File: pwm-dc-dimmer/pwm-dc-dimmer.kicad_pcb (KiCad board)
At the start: 2 copper layers, 61 x 125.5 mm, 90 parts, among them J1 Screw_Terminal_01x02, J10 Screw_Terminal_01x02, J11 Screw_Terminal_01x02, J12 Screw_Terminal_01x02, J13 Screw_Terminal_01x02, J14 Conn_02x03_Odd_Even, J15 Conn_02x03_Odd_Even, J2 Screw_Terminal_01x02, J3 Screw_Terminal_01x02, J4 Screw_Terminal_01x02, J5 Screw_Terminal_01x02, J6 Screw_Terminal_01x02, J7 Screw_Terminal_01x02, J8 Screw_Terminal_01x02, J9 Screw_Terminal_01x02, Q1 Q_NMOS_GDS, Q10 Q_NMOS_GDS, Q11 Q_NMOS_GDS, Q12 Q_NMOS_GDS, Q2 Q_NMOS_GDS, Q3 Q_NMOS_GDS, Q4 Q_NMOS_GDS, Q5 Q_NMOS_GDS, Q6 Q_NMOS_GDS, Q7 Q_NMOS_GDS, Q8 Q_NMOS_GDS, Q9 Q_NMOS_GDS

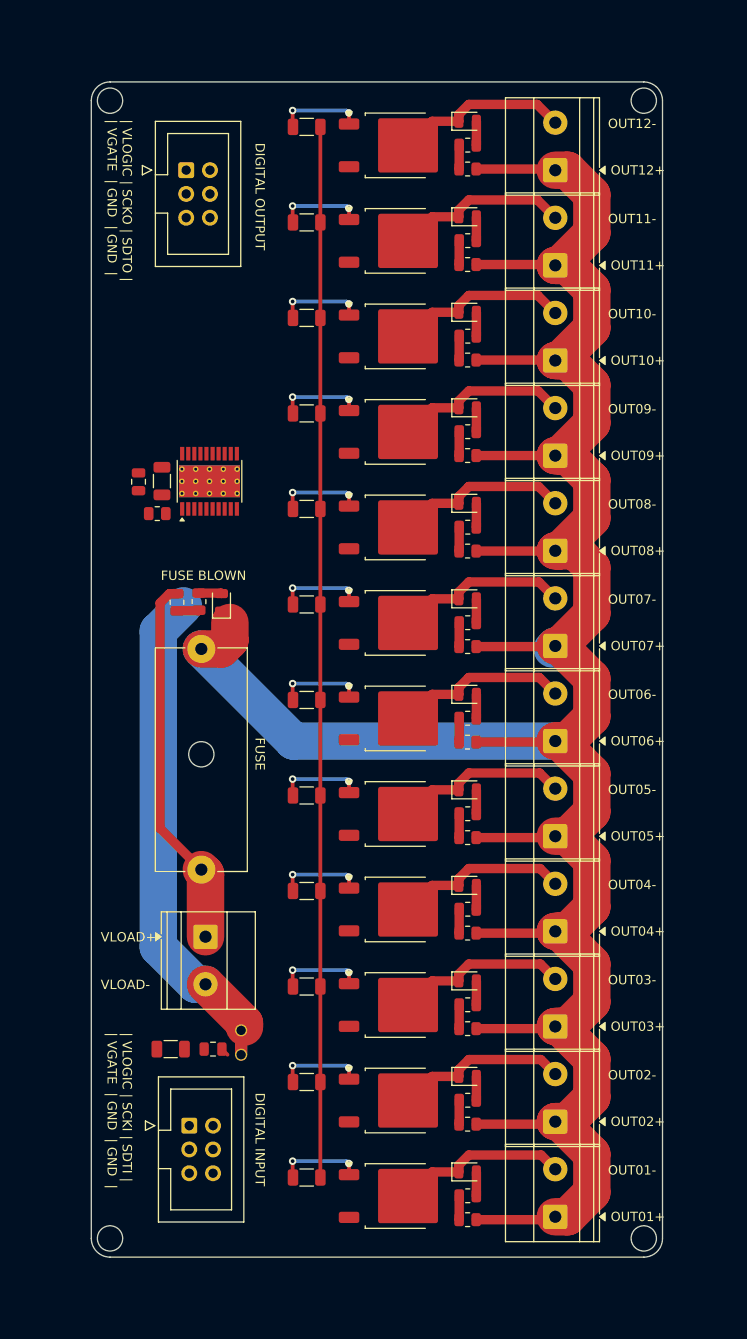
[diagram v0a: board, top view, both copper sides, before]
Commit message: Finish routing
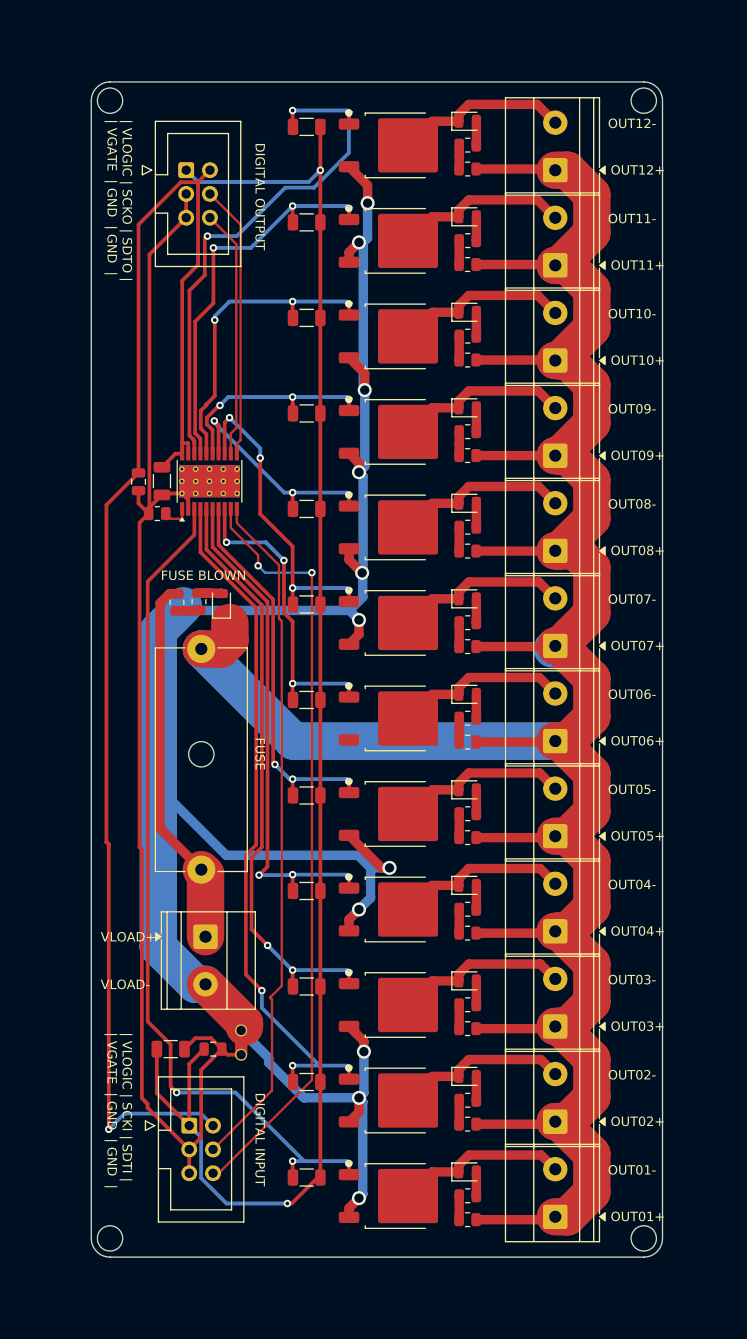
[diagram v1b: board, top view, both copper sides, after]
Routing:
- net GND_LOAD: track 50.5 -> 218.4 mm, vias 0 -> 11
- net GND: track 0.85 -> 157.0 mm
- net V_LOGIC: track 0.00 -> 155.1 mm, vias 0 -> 1
- net GATE_SINK_1: track 9.07 -> 91.9 mm, vias 2 -> 3
- net SDTI: track 0.00 -> 82.2 mm, vias 0 -> 2
- net SCKI: track 0.00 -> 73.8 mm
- net GATE_SINK_2: track 9.07 -> 74.7 mm, vias 2 -> 3
- net V_GATE: track 113.1 -> 173.4 mm, vias 0 -> 2
- net GATE_SINK_3: track 9.07 -> 63.1 mm, vias 2 -> 3
- net GATE_SINK_12: track 9.07 -> 56.6 mm, vias 2 -> 3
- net GATE_SINK_4: track 9.07 -> 55.1 mm, vias 2 -> 3
- net GATE_SINK_11: track 9.07 -> 42.4 mm, vias 2 -> 3
- net GATE_SINK_5: track 9.07 -> 41.4 mm, vias 2 -> 3
- net SCKO: track 0.00 -> 29.3 mm
- net SDTO: track 0.00 -> 26.6 mm
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
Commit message: Finalize DC dimmer v0.1
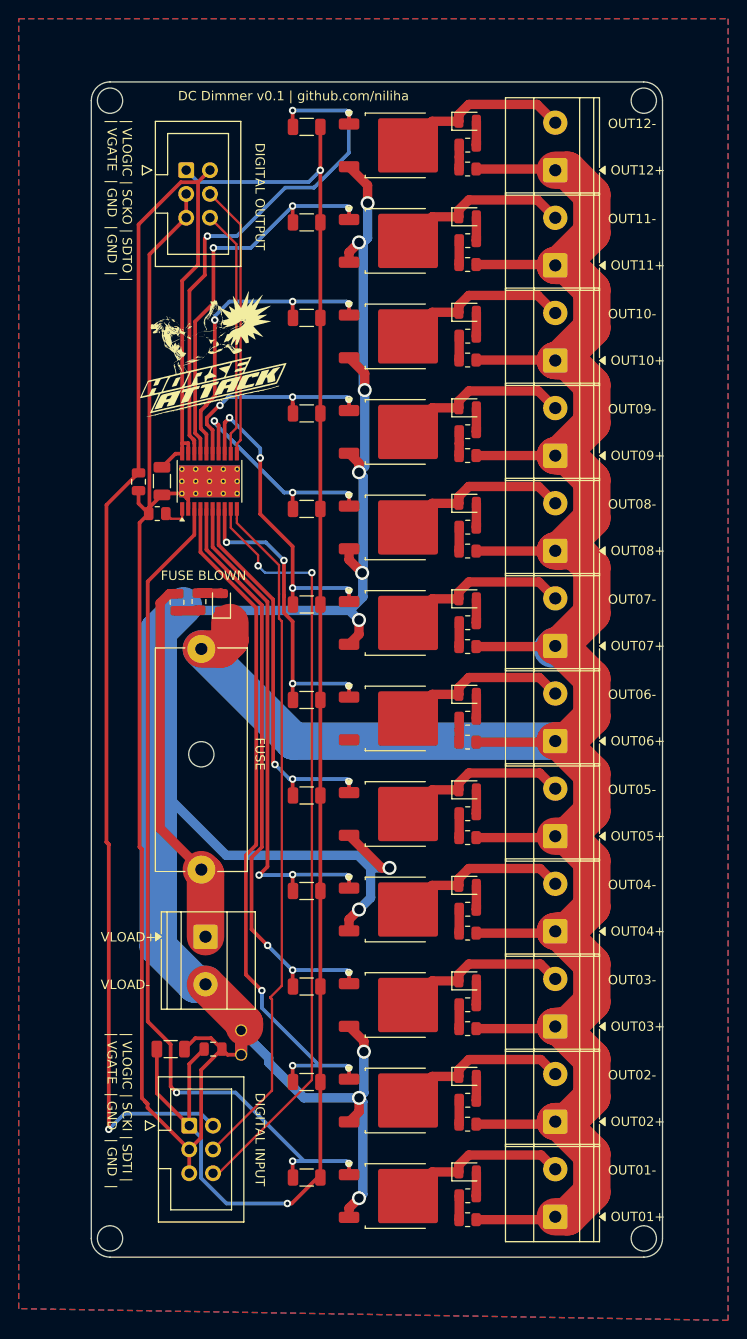
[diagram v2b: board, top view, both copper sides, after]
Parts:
- added G***: LOGO, LOGO, F.Cu at (95.5, 85.8)
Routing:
- added copper zone on B.Cu, net GND
- added copper zone on F.Cu, net GND
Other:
- board text added: "DC Dimmer v0.1 | github.com/niliha"
- board text added: "JLCJLCJLCJLC"
